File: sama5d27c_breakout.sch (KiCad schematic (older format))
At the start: 1 part, among them U1 SAMA5D2x-SIP

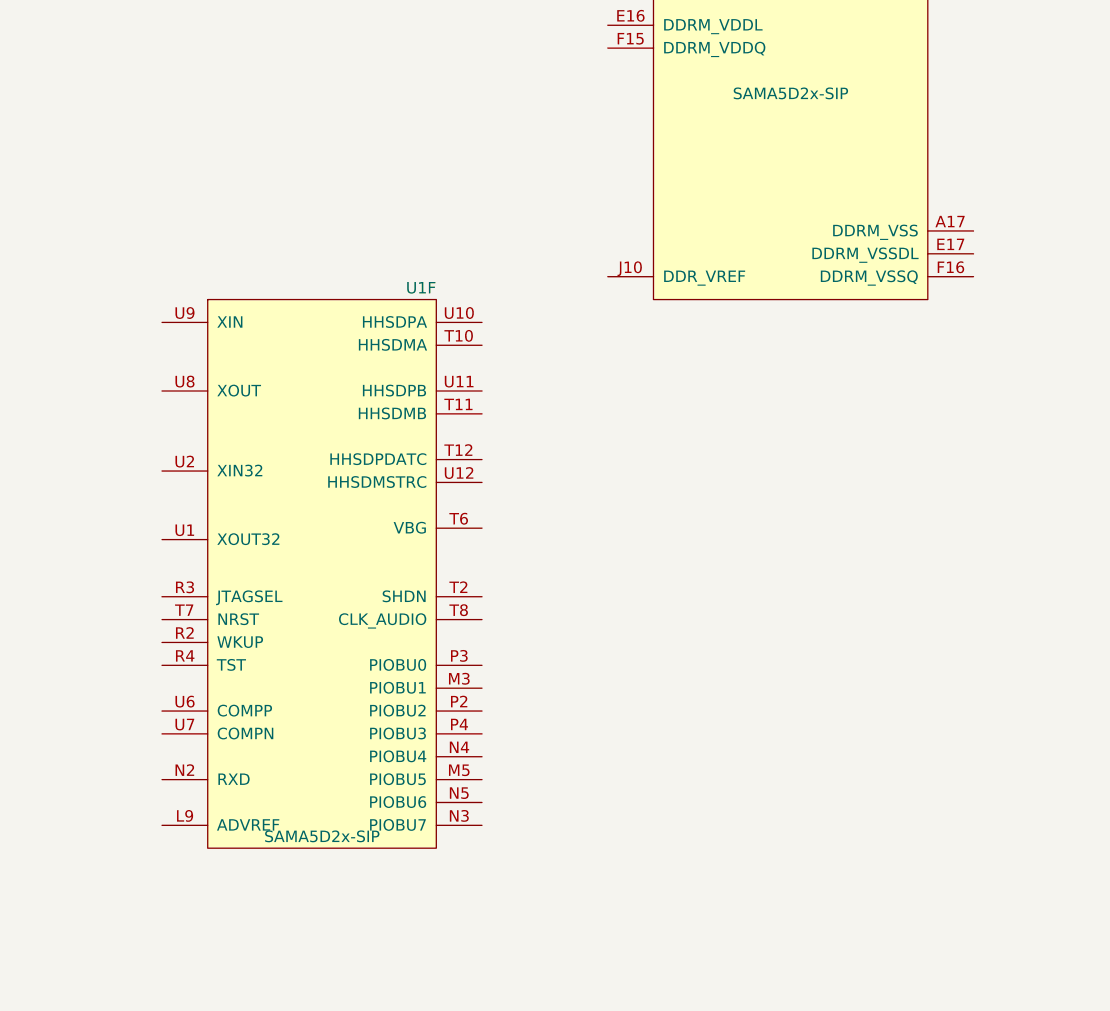
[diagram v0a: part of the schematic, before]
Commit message: Connected Unit F
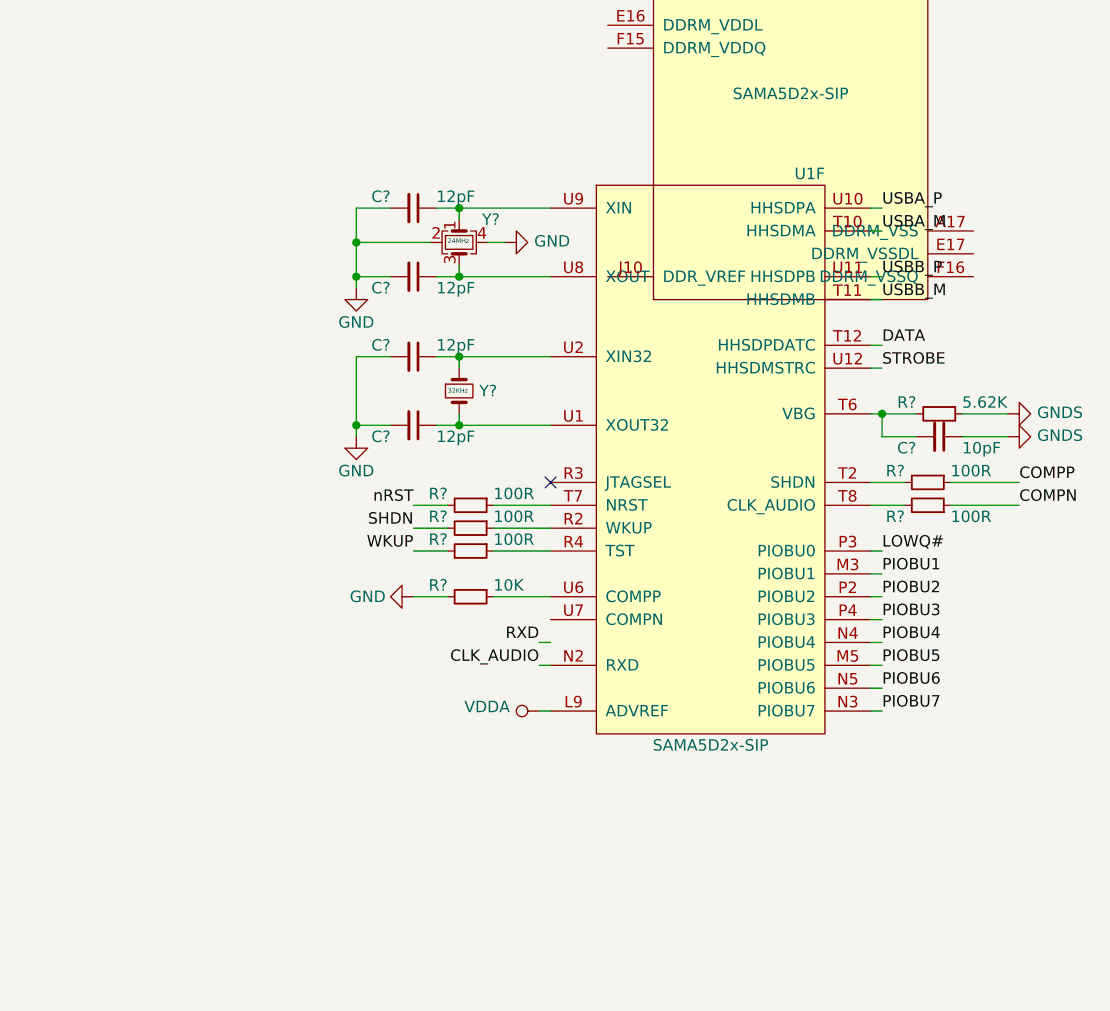
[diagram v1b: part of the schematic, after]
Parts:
- added C?: 10pF, symbol Device:C_Small
- added C? (x4): 12pF, symbol Device:C_Small
- added R? (x5): 100R, symbol Device:R_Small
- added R?: 5.62K, symbol Device:R_Small
- added R?: 10K, symbol Device:R_Small
- added Y?: NX2016SA_24MHz, symbol Device:Crystal_GND24_Small
- added Y?: NX2012SA_32-768KHz, symbol Device:Crystal_Small
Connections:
- net VDDA: now reaches U1.L9 (ADVREF)
- net PIOBU1: now reaches U1.M3 (PIOBU1)
- net PIOBU5: now reaches U1.M5 (PIOBU5)
- net CLK_AUDIO: now reaches U1.N2 (RXD)
- net PIOBU7: now reaches U1.N3 (PIOBU7)
- net PIOBU4: now reaches U1.N4 (PIOBU4)
- net PIOBU6: now reaches U1.N5 (PIOBU6)
- net PIOBU2: now reaches U1.P2 (PIOBU2)
- net LOWQ#: now reaches U1.P3 (PIOBU0)
- net PIOBU3: now reaches U1.P4 (PIOBU3)
- net at U1.R2 (WKUP): now also R?.1
- net at U1.R4 (TST): now also R?.1
- net USBA_M: now reaches U1.T10 (HHSDMA)
- net USBB_M: now reaches U1.T11 (HHSDMB)
- net DATA: now reaches U1.T12 (HHSDPDATC)
- net at U1.T2 (SHDN): now also R?.2
- net at U1.T6 (VBG): now also C?.2, R?.2
- net at U1.T7 (NRST): now also R?.1
- net at U1.T8 (CLK_AUDIO): now also R?.2
- net at U1.U1 (XOUT32): now also C?.1, Y?.2
- net USBA_P: now reaches U1.U10 (HHSDPA)
- net USBB_P: now reaches U1.U11 (HHSDPB)
- net STROBE: now reaches U1.U12 (HHSDMSTRC)
- net at U1.U2 (XIN32): now also C?.1, Y?.1
- net at U1.U6 (COMPP): now also R?.1
- net at U1.U8 (XOUT): now also C?.1, Y?.3
- net at U1.U9 (XIN): now also C?.1, Y?.1
- new net COMPN: R?.1
- new net COMPP: R?.1
- new net GND: C?.2, C?.2, C?.2, C?.2, R?.2, Y?.2, Y?.4
- new net GNDS: C?.1, R?.1
- new net SHDN: R?.2
- new net WKUP: R?.2
- new net nRST: R?.2
- no-connect marks 0 -> 1
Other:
- note added: "24MHz"
- note added: "32KHz"
- moved on the sheet: U1F
